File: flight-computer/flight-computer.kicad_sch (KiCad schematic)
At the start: 32 parts, among them J1 Conn_01x06_Pin, J2 Conn_01x06_Pin, J3 Power Connector, J4 Micro_SD_Card, J5 USB_C_Receptacle_USB2.0_16P, J6 Conn_01x02_Pin, Q1 DMN3404L, Q2 DMN3404L, SW1 Reset, SW2 Boot, U1 LMR51420X, U2 ESP32-S3-WROOM-1, U3 LSM6DSO32TR

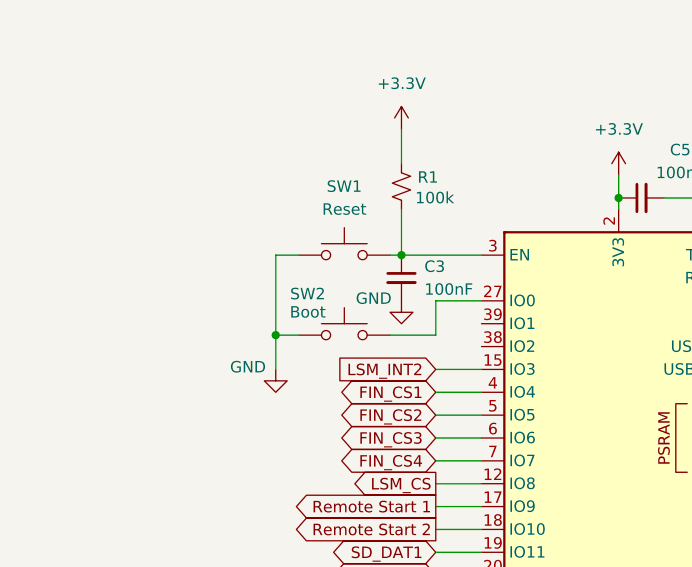
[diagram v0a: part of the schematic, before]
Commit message: finishing(?) touches on flight computer board
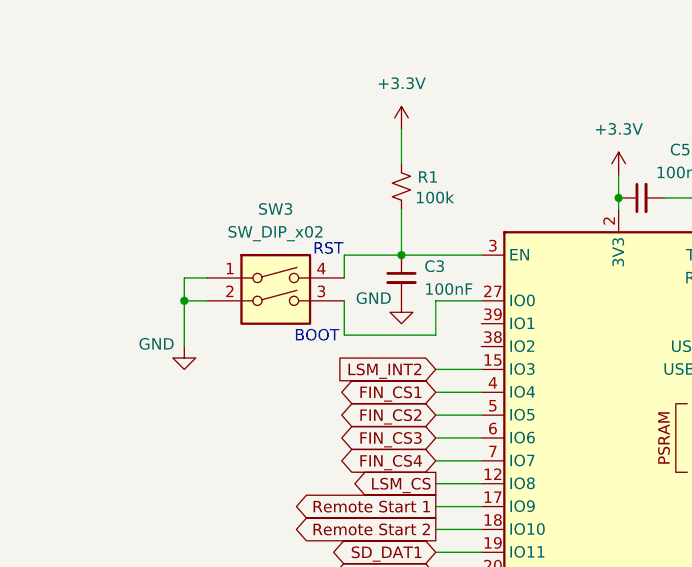
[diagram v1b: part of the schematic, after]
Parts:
- removed SW1: Reset, Jumper:SolderJumper-2_P1.3mm_Open_RoundedPad1.0x1.5mm, symbol Switch:SW_Push
- removed SW2: Boot, Library:SW_FSM2JMTR_TEC, symbol Switch:SW_Push
- added SW3: SW_DIP_x02, Library:218-2LPSTR_CTS, symbol Switch:SW_DIP_x02
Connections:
- net GND: now also SW3.1, SW3.2
- net at C3.1, R1.2, U2.3 (EN): now also SW3.4
- net at U2.27 (IO0): now also SW3.3
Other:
- note added: "BOOT"
- note added: "RST"
